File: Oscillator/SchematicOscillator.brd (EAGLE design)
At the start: 85.1 x 32.7 mm, 22 parts, among them X1 BU-SMA-H, X2 BU-SMA-H

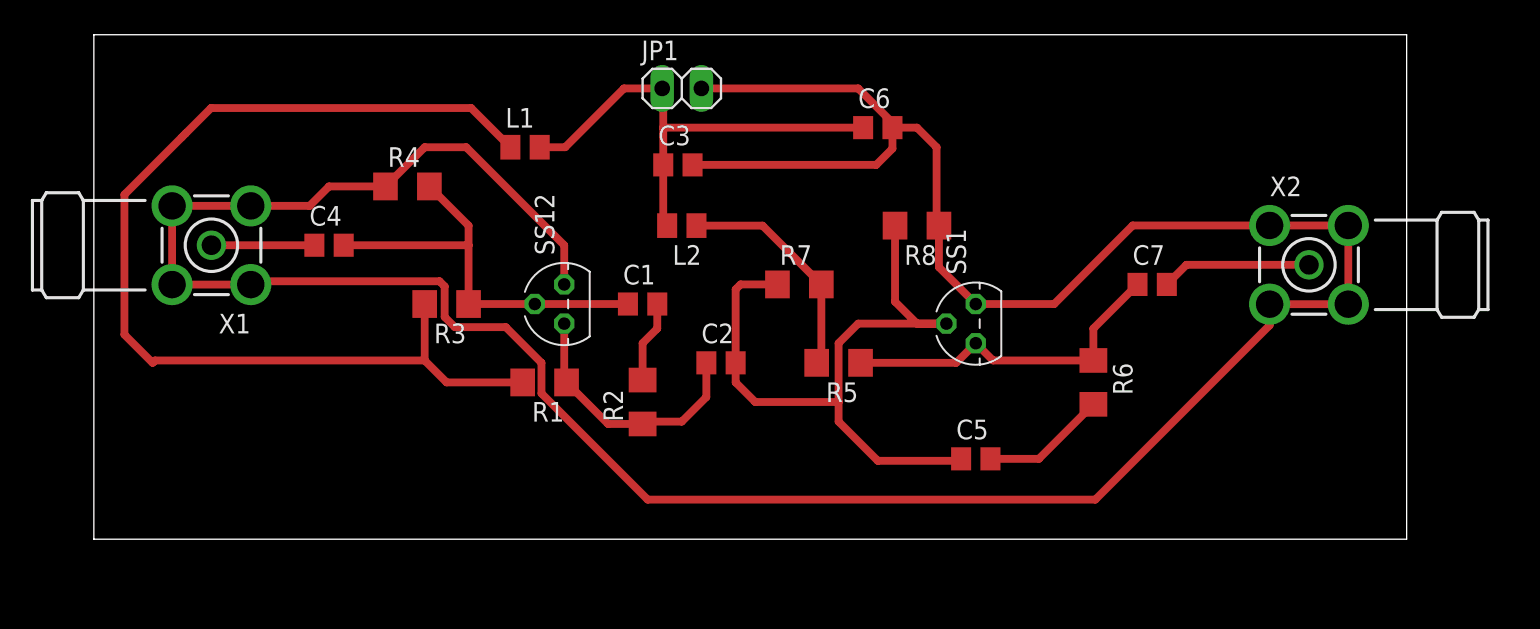
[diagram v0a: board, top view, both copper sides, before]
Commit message: Ocillator File - PCB
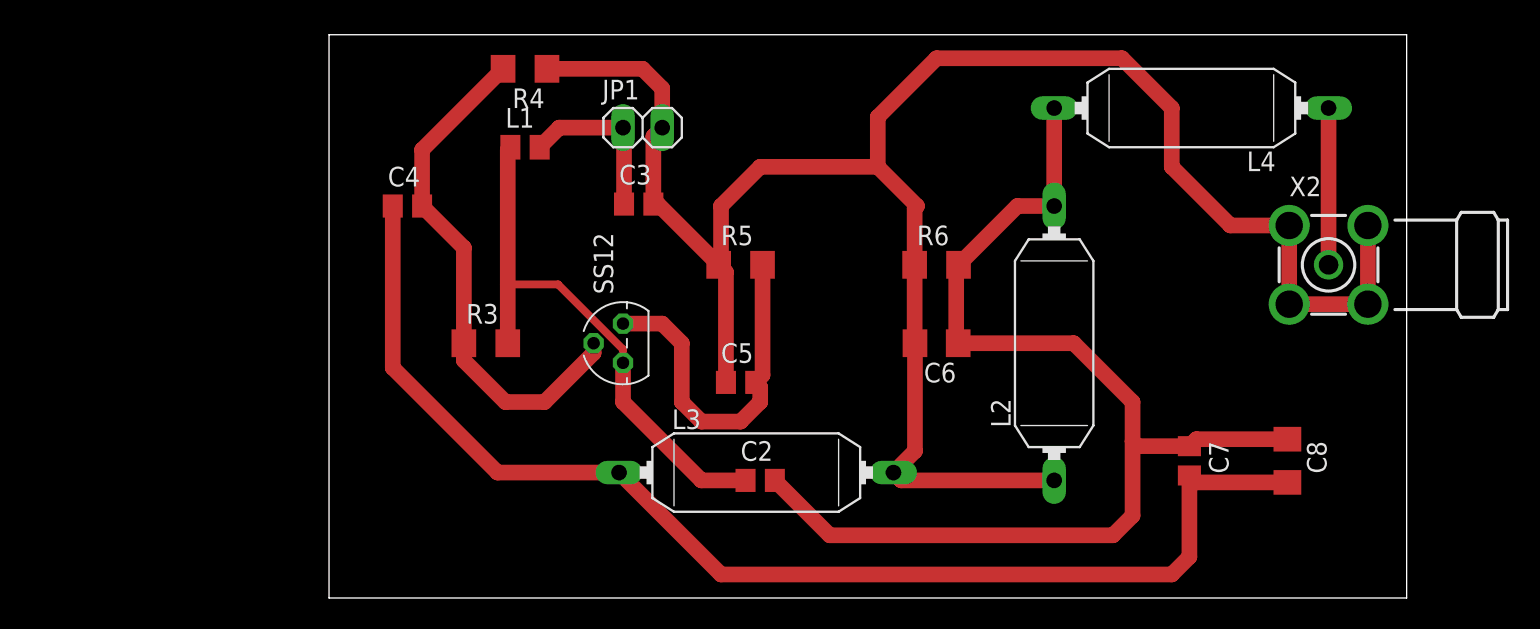
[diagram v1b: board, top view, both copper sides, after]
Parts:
- removed C1: 0.1u, rcl:C0805
- removed R1, R2, R7, R8: (no value), rcl:R1206
- removed SS1: (no value), transistor:TO92
- removed X1: BU-SMA-H, con-coax:BU-SMA-H
- added C8: 4p, rcl:C1206
- added L3, L4: B82131, inductors:SUKW1-17
- C6: value 0.1u -> 4p; device rcl:C0805 -> rcl:C1206
- C7: value 0.1u -> 22p
- L2: value (none) -> B82131; device resistor:M0805 -> inductors:SUKW1-17
- moved L2 25.3 mm to (61.0, 83.8), turned to 90 degrees
- moved C5 16.0 mm to (40.6, 81.3)
- moved C6 14.5 mm to (53.3, 83.8), turned to 180 degrees
- moved R6 12.7 mm to (53.3, 88.9), turned to 0 degrees
- moved C7 11.7 mm to (69.7, 76.2), turned to 270 degrees
- moved R4 10.8 mm to (26.7, 101.6), turned to 180 degrees
- moved R5 8.98 mm to (40.6, 88.9), turned to 0 degrees
- moved C2 8.03 mm to (41.9, 74.9)
- moved C4 5.68 mm to (19.1, 92.7)
- moved SS12 4.58 mm to (33.0, 83.8)
- moved R3 3.59 mm to (24.1, 83.8), turned to 0 degrees
- moved C3 3.59 mm to (34.0, 92.8)
- moved JP1 3.59 mm to (34.3, 97.8)
- moved X2 1.27 mm to (78.7, 88.9)
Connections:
- removed net N$1: C1.2, R2.2
- removed net N$10: C5.2, R6.2
- removed net N$11: C7.2, X2.1
- removed net N$3: C2.1, R1.1, R2.1, SS12.3
- removed net N$9: C2.2, C5.1, R7.1, R8.2, SS1.2
- new net N$6: L4.1, X2.1
- net GND: now also C5.1, L2.1, L3.2, R5.1, R6.1; no longer R8.1, SS1.1, SS12.1, X1.2, X1.3, X1.4, X1.5
- net N$2: now also C2.1, SS12.3; no longer R1.2
- net N$4: now also C5.2, R5.2, SS12.1; no longer C4.1, X1.1
- net N$5: no longer C1.1
- net N$7: now also C2.2, C6.1, C7.1, C8.1, L2.2, L4.2, R6.2; no longer L2.1, R5.2, R7.2
- net N$8: now also C4.1, C7.2, C8.2, L3.1; no longer C7.1, R5.1, R6.1, SS1.3
- net VCC: no longer C6.1, L2.2
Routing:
- net GND: track 202.5 -> 130.1 mm
- net N$7: track 14.9 -> 75.2 mm
- net N$8: track 22.2 -> 79.9 mm
- net N$9: track 46.5 -> 0.00 mm
- net N$2: track 68.7 -> 35.4 mm
- net VCC: track 32.5 -> 10.9 mm
- net N$3: track 17.0 -> 0.00 mm
- net N$4: track 6.67 -> 23.5 mm
- net N$6: track 0.00 -> 10.2 mm
- net N$11: track 9.74 -> 0.00 mm
- net N$10: track 8.13 -> 0.00 mm
- net N$5: track 27.1 -> 33.7 mm
- net N$1: track 5.32 -> 0.00 mm
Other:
- board size 85.1 x 32.7 mm -> 69.8 x 36.5 mm
